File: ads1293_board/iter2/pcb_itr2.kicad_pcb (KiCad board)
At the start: 2 copper layers, 23.5 x 28.1 mm, 28 parts, among them J1 Conn_01x05_Pin, J2 RSTB_J, J3 Breakout Pins, J4 Power Input, U1 ADS1293CISQ/NOPB, U2 SPX5205M5-L-5-0/TR, Y1 4.096 MHz

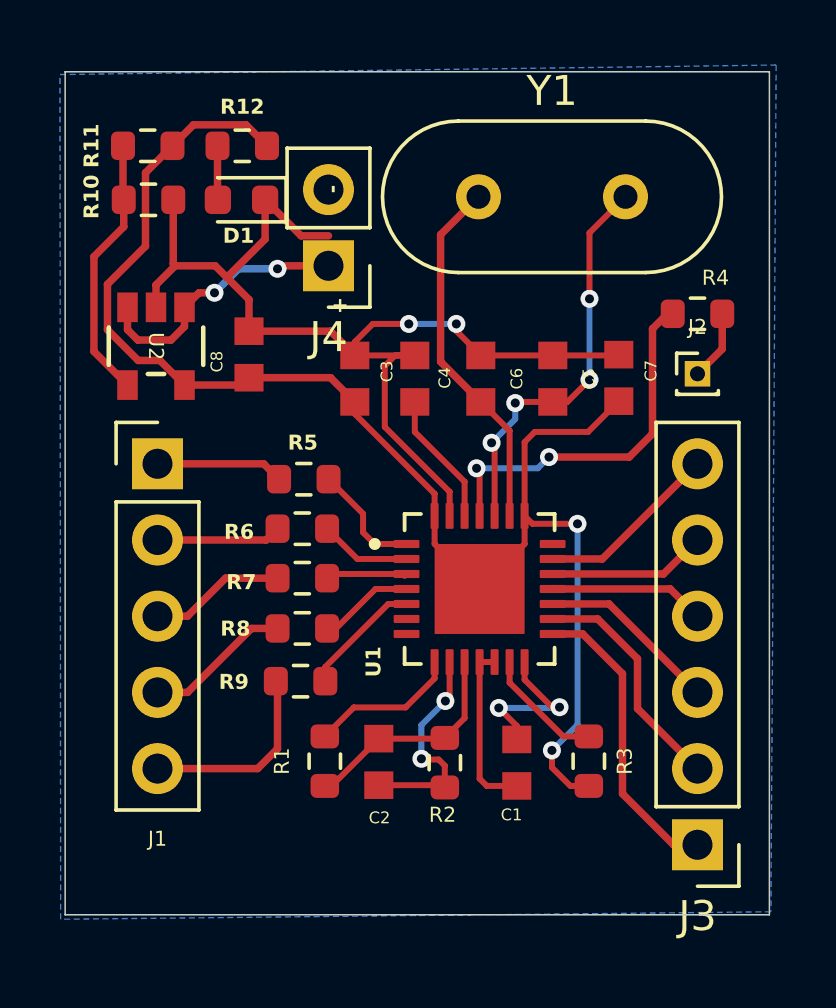
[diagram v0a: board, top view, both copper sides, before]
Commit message: more docs
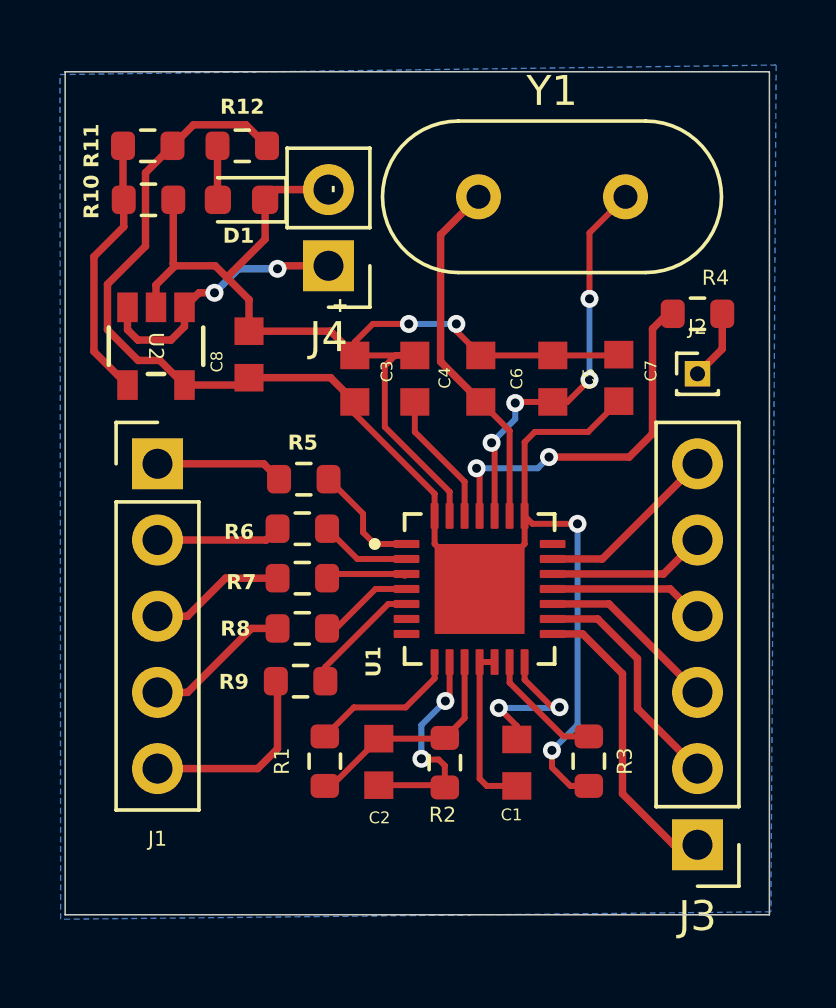
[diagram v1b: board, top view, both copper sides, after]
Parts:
- R10: value 22K Ohm -> 12K Ohm
- R11: value 12K Ohm -> 22K Ohm
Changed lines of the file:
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@@
 			)
 		)
-		(property "Value" "12K Ohm"
+		(property "Value" "22K Ohm"
 			(at 0 1.43 0)
 			(layer "F.Fab")
@@
 			)
 		)
-		(property "Value" "22K Ohm"
+		(property "Value" "12K Ohm"
 			(at 0 1.43 0)
 			(layer "F.Fab")
@@
 	)
 	(segment
-		(start 124.2875 70.4)
-		(end 123.0875 69.2)
-		(width 0.25)
-		(layer "F.Cu")
-		(net 5)
-	)
-	(segment
 		(start 129.23666 78.93196)
 		(end 129.23666 79.737646)
@@
 	)
 	(segment
+		(start 125.2 68.86)
+		(end 123.4275 68.86)
+		(width 0.25)
+		(layer "F.Cu")
+		(net 5)
+	)
+	(segment
+		(start 123.4275 68.86)
+		(end 123.0875 69.2)
+		(width 0.25)
+		(layer "F.Cu")
+		(net 5)
+	)
+	(segment
 		(start 120.088899 71.4)
 		(end 121.425 71.4)
@@
 	)
 	(segment
+		(start 125.2 68.86)
+		(end 125.86 68.86)
+		(width 0.25)
+		(layer "F.Cu")
+		(net 5)
+	)
+	(segment
 		(start 132.652395 86.113381)
 		(end 131.73666 85.197646)
@@
 		(net 5)
 	)
-	(segment
-		(start 125.2 70.4)
-		(end 124.2875 70.4)
-		(width 0.25)
-		(layer "F.Cu")
-		(net 5)
-	)
 	(via
 		(at 132.900925 86.113381)
@@
 	)
 	(segment
-		(start 118.35 69.175)
-		(end 118.375 69.2)
+		(start 117.382098 71.092902)
+		(end 117.382098 74.2571)
 		(width 0.25)
 		(layer "F.Cu")
@@
 	)
 	(segment
-		(start 117.382098 71.092902)
-		(end 117.382098 74.2571)
+		(start 118.35 67.4)
+		(end 118.35 69.175)
 		(width 0.25)
 		(layer "F.Cu")
@@
 	)
 	(segment
-		(start 118.35 67.4)
-		(end 118.35 69.175)
+		(start 118.35 69.175)
+		(end 118.375 69.2)
 		(width 0.25)
 		(layer "F.Cu")
